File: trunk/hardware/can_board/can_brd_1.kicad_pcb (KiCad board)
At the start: 2 copper layers, 23.3 x 10.9 mm, 11 parts, among them P451 CONN_4, P452 CONN_2, U451 SN65HVD230

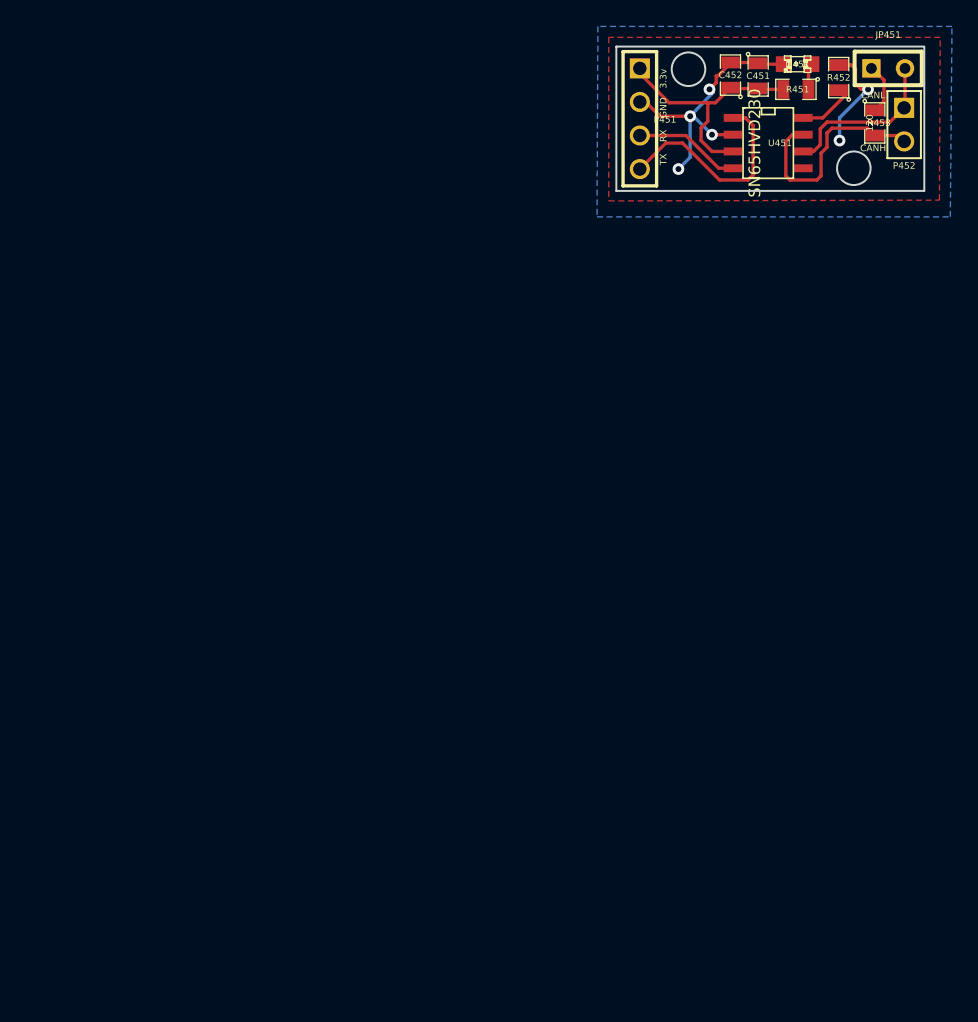
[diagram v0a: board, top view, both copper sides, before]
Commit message: new location
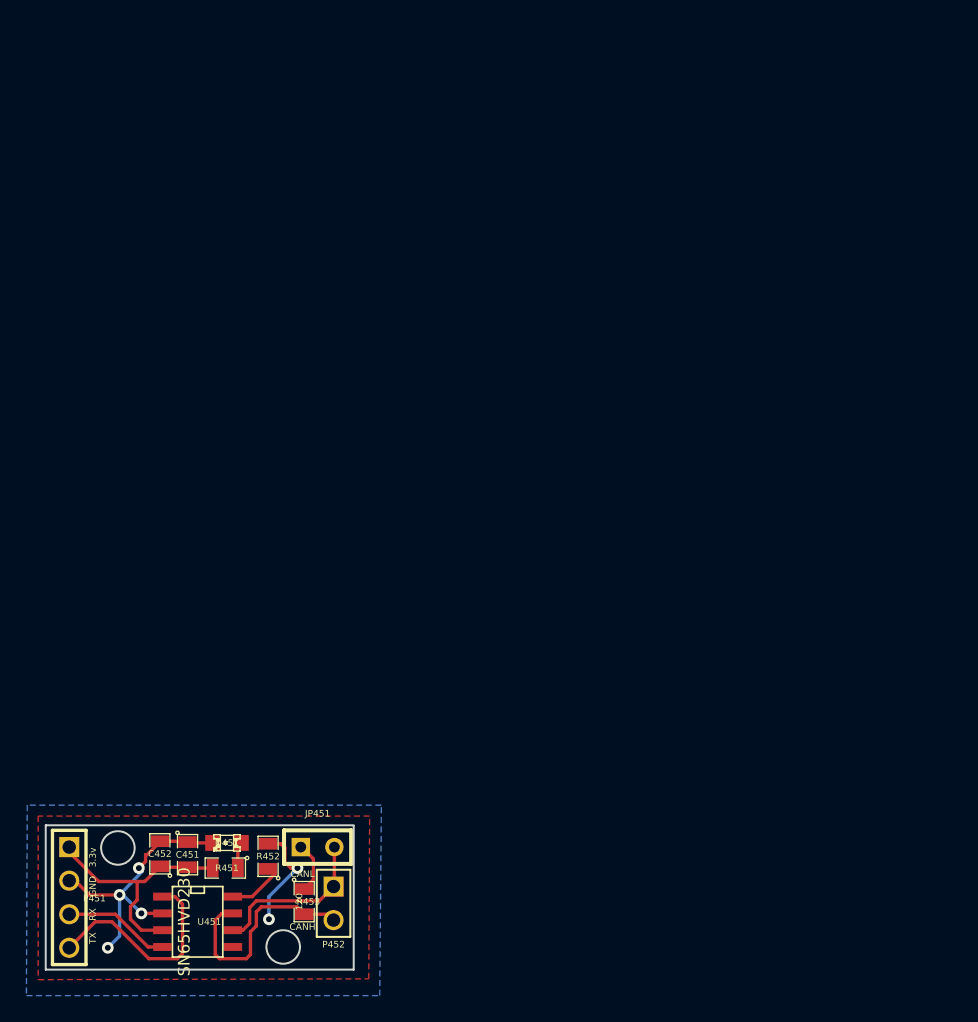
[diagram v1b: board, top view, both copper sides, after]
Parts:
- moved C451 73.1 mm to (145.5, 180.1)
- moved C452 73.1 mm to (143.4, 180.0)
- moved P452 73.1 mm to (156.5, 183.8)
- moved D451 73.1 mm to (148.5, 179.2)
- moved G451 73.1 mm to (145.8, 183.5)
- moved JP451 73.1 mm to (155.3, 179.5)
- moved P451 73.1 mm to (136.5, 183.3)
- moved R452 73.1 mm to (151.6, 180.2)
- moved R453 73.1 mm to (154.3, 183.6)
- moved U451 73.1 mm to (146.2, 185.2)
- moved R451 73.1 mm to (148.3, 181.1)
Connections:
- net /RX renamed /CAN_RX
- net /TX renamed /CAN_TX
